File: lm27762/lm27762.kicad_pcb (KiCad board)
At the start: 2 copper layers, 17.9 x 14.1 mm, 13 parts, among them J1 Conn_01x04

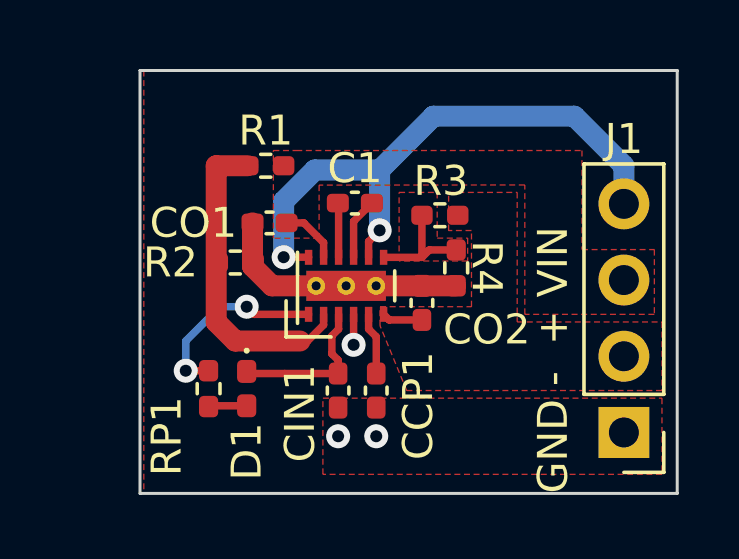
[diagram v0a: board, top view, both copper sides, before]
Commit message: updated design files to RevA
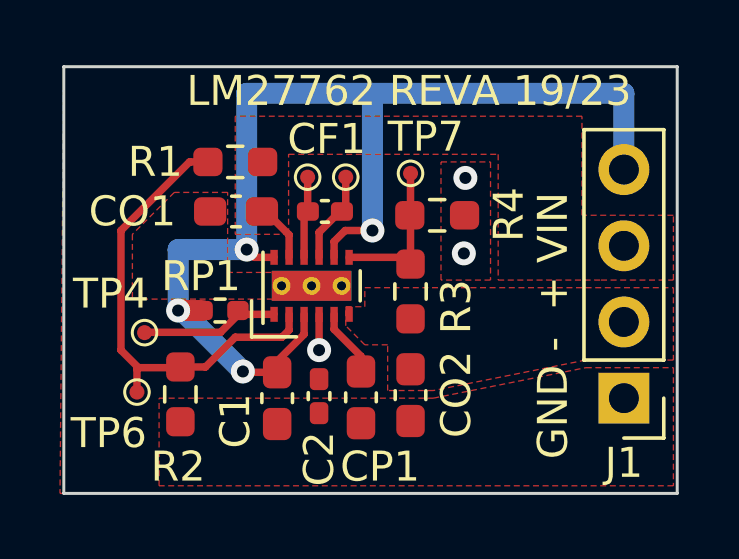
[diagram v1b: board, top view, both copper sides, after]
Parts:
- removed CCP1, CIN1: 1u, Capacitor_SMD:C_0402_1005Metric_Pad0.74x0.62mm_HandSolder
- removed D1: LED, LED_SMD:LED_0402_1005Metric_Pad0.77x0.64mm_HandSolder
- added C2: 1u, Capacitor_SMD:C_0402_1005Metric_Pad0.74x0.62mm_HandSolder, F.Cu at (116.5, 67.2)
- added CF1: 1u, Capacitor_SMD:C_0402_1005Metric_Pad0.74x0.62mm_HandSolder, F.Cu at (116.7, 61.1)
- added CP1: 4.7u, Capacitor_SMD:C_0603_1608Metric_Pad1.08x0.95mm_HandSolder, F.Cu at (117.9, 67.3)
- added TP2: TestPoint, TinyTestPoints:0_5mm, F.Cu at (117.3, 59.9)
- added TP3: TestPoint, TinyTestPoints:0_5mm, F.Cu at (116.1, 59.9)
- added TP4: TestPoint, TinyTestPoints:0_5mm, F.Cu at (110.6, 65.1)
- added TP6: TestPoint, TinyTestPoints:0_5mm, F.Cu at (110.4, 67.1)
- added TP7: TestPoint, TinyTestPoints:0_5mm, F.Cu at (119.5, 59.8)
- C1: value 1u -> 10u; footprint Capacitor_SMD:C_0402_1005Metric_Pad0.74x0.62mm_HandSolder -> Capacitor_SMD:C_0603_1608Metric_Pad1.08x0.95mm_HandSolder
- CO1, CO2: value 1u -> 2.2u; footprint Capacitor_SMD:C_0402_1005Metric_Pad0.74x0.62mm_HandSolder -> Capacitor_SMD:C_0603_1608Metric_Pad1.08x0.95mm_HandSolder
- R1, R3: value ~ -> 680k; footprint Resistor_SMD:R_0402_1005Metric_Pad0.72x0.64mm_HandSolder -> Resistor_SMD:R_0603_1608Metric_Pad0.98x0.95mm_HandSolder
- R2, R4: value ~ -> 220k; footprint Resistor_SMD:R_0402_1005Metric_Pad0.72x0.64mm_HandSolder -> Resistor_SMD:R_0603_1608Metric_Pad0.98x0.95mm_HandSolder
- U1: value ~ -> LM27762DSSR
- moved C1 7.00 mm to (115.1, 67.3), turned to -90 degrees
- moved R2 4.76 mm to (111.8, 67.2), turned to 90 degrees
- moved CO2 3.10 mm to (119.5, 67.2), turned to -90 degrees
- moved R3 2.72 mm to (119.5, 63.8), turned to 90 degrees
- moved RP1 2.63 mm to (113.2, 64.4), turned to 180 degrees
- moved R4 1.86 mm to (120.4, 61.2), turned to 0 degrees
- moved CO1 1.18 mm to (113.7, 61.1)
- moved U1 1.15 mm to (116.2, 63.6)
- moved J1 1.14 mm to (126.6, 67.3)
- moved R1 1.02 mm to (113.7, 59.4)
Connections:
- C1 pad 1: Net-(U1-C1+) -> /VIN
- C1 pad 2: Net-(U1-C1-) -> GND
- RP1 pad 2: Net-(D1-A) -> /VIN
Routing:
- net /VIN: track 25.5 -> 39.4 mm, vias 2 -> 4
- net GND: track 7.50 -> 1.19 mm
- net /fb+: track 10.7 -> 15.5 mm
- net Net-(U1-PGOOD): track 6.43 -> 4.55 mm, vias 2 -> 0
- net Net-(D1-A): track 1.28 -> 0.00 mm
- net /VOUT-: track 1.28 -> 0.00 mm
- net /fb-: track 3.93 -> 5.15 mm
- net Net-(U1-C1-): track 2.06 -> 3.04 mm
- net Net-(U1-C1+): track 1.82 -> 2.72 mm
- removed copper zone on F.Cu, net /fb-
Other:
- board size 17.9 x 14.1 mm -> 20.4 x 14.2 mm
- board text added: "LM27762 REVA 19/23"
- board text added: "TP4"
- board text added: "TP6"
- board text added: "TP7"
